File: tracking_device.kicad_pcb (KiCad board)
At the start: 4 copper layers, 74.2 x 35 mm, 74 parts, among them J1 USB_OTG, J2 CONN_COAXIAL, J3 JST-PH, J4 Micro_SD_Connector, J5 CONN_01X03, J6 CONN_01X06, J7 CONN_01X03, J8 SMA, Q1 PMGD280UN, SW1 SW_Push, U1 RClamp0503F, U2 LDK220M30R, U3 MCP73831, U4 MAX-M8, U5 STC3100, U6 STM32L476RG, U7 RFM95W, Y1 ABS07-120-32.768kHz-T

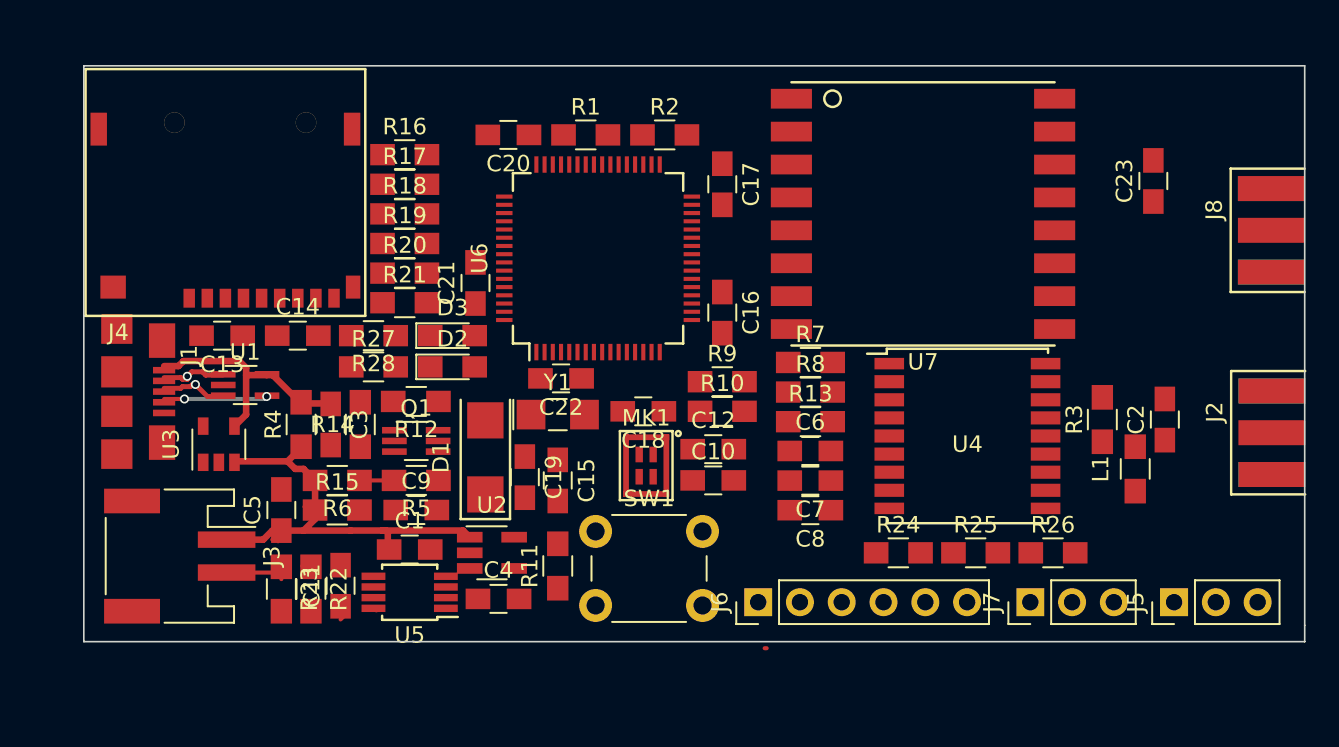
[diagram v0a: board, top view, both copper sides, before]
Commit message: Version sent out for fabrication
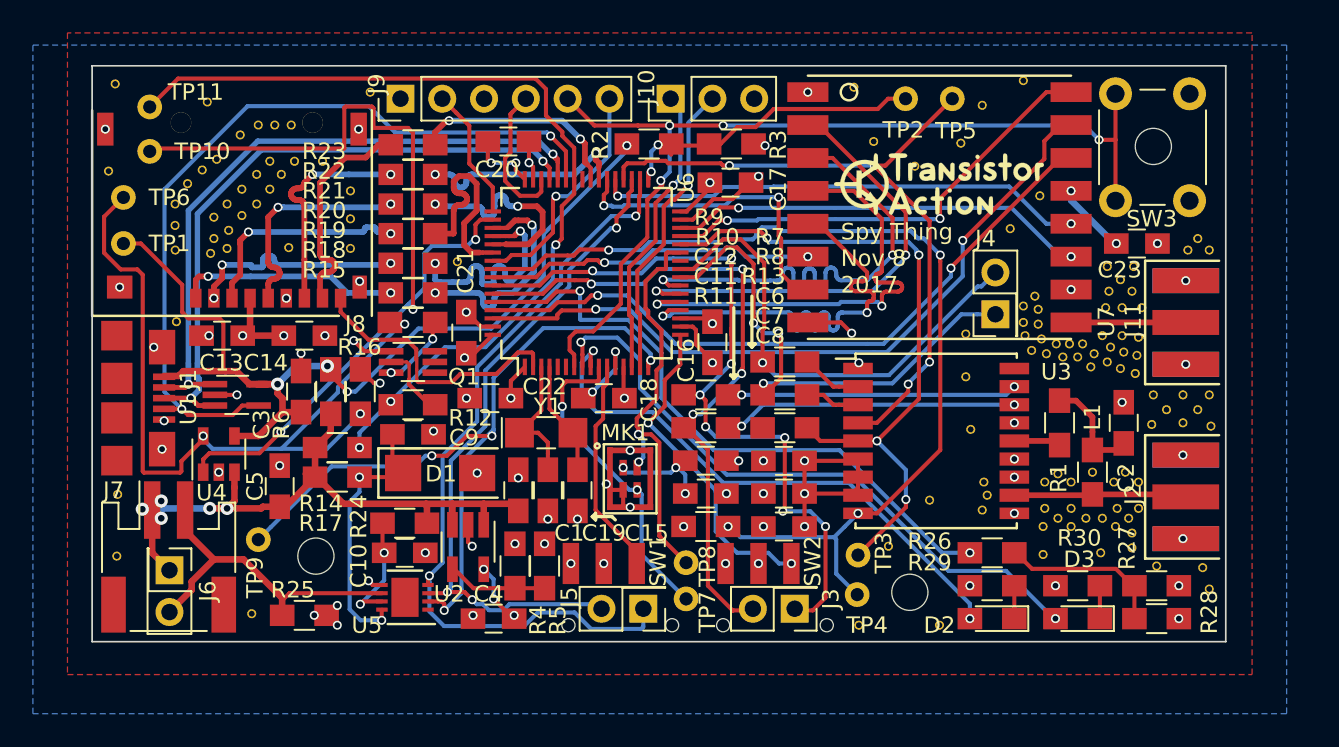
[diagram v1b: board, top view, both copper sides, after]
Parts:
- added ?: , tracking_device:VIA_0.35mm_0.55mm, F.Cu at (97.6, 95.5)
- added ?: , tracking_device:VIA_0.35mm_0.55mm, F.Cu at (155.8, 92.2)
- added ?: , tracking_device:VIA_0.35mm_0.55mm, F.Cu at (154.3, 93.7)
- added ?: , tracking_device:VIA_0.35mm_0.55mm, F.Cu at (154.1, 94.7)
- added ?: , tracking_device:VIA_0.35mm_0.55mm, F.Cu at (153.2, 98.3)
- added ?: , tracking_device:VIA_0.35mm_0.55mm, F.Cu at (152.4, 97.7)
- added ?: , tracking_device:VIA_0.35mm_0.55mm, F.Cu at (151.5, 97.7)
- added ?: , tracking_device:VIA_0.35mm_0.55mm, F.Cu at (150.5, 97.5)
- added ?: , tracking_device:VIA_0.35mm_0.55mm, F.Cu at (149.6, 97.3)
- added ?: , tracking_device:VIA_0.35mm_0.55mm, F.Cu at (149.2, 96.4)
- added ?: , tracking_device:VIA_0.35mm_0.55mm, F.Cu at (149.1, 95.6)
- added ?: , tracking_device:VIA_0.35mm_0.55mm, F.Cu at (149.1, 94.6)
- added ?: , tracking_device:VIA_0.35mm_0.55mm, F.Cu at (155.0, 93.0)
- added ?: , tracking_device:VIA_0.35mm_0.55mm, F.Cu at (149.8, 94.0)
- added ?: , tracking_device:VIA_0.35mm_0.55mm, F.Cu at (150.0, 94.8)
- added ?: , tracking_device:VIA_0.35mm_0.55mm, F.Cu at (150.0, 95.7)
- added ?: , tracking_device:VIA_0.35mm_0.55mm, F.Cu at (150.2, 96.6)
- added ?: , tracking_device:VIA_0.35mm_0.55mm, F.Cu at (151.1, 96.9)
- added ?: , tracking_device:VIA_0.35mm_0.55mm, F.Cu at (151.9, 96.9)
- added ?: , tracking_device:VIA_0.35mm_0.55mm, F.Cu at (152.7, 96.9)
- added ?: , tracking_device:VIA_0.35mm_0.55mm, F.Cu at (155.0, 98.4)
- added ?: , tracking_device:VIA_0.35mm_0.55mm, F.Cu at (153.4, 97.5)
- added ?: , tracking_device:VIA_0.35mm_0.55mm, F.Cu at (154.2, 98.0)
- added ?: , tracking_device:VIA_0.35mm_0.55mm, F.Cu at (155.7, 93.7)
- added ?: , tracking_device:VIA_0.35mm_0.55mm, F.Cu at (155.9, 98.7)
- added ?: , tracking_device:VIA_0.35mm_0.55mm, F.Cu at (154.4, 97.1)
- added ?: , tracking_device:VIA_0.35mm_0.55mm, F.Cu at (153.9, 96.4)
- added ?: , tracking_device:VIA_0.35mm_0.55mm, F.Cu at (155.2, 97.4)
- added ?: , tracking_device:VIA_0.35mm_0.55mm, F.Cu at (104.5, 91.0)
- added ?: MOUNTING_HOLE, Mounting_Holes:MountingHole_2.2mm_M2, F.Cu at (106.1, 109.8)
- added ?: MOUNTING_HOLE, Mounting_Holes:MountingHole_2.2mm_M2, F.Cu at (142.2, 112.0)
- added ?: MOUNTING_HOLE, Mounting_Holes:MountingHole_2.2mm_M2, F.Cu at (157.0, 84.9)
- added ?: , tracking_device:VIA_0.35mm_0.55mm, F.Cu at (156.0, 97.6)
- added ?: LOGO, tracking_device:logo_2, F.Cu at (144.0, 87.1)
- added ?: , tracking_device:VIA_0.35mm_0.55mm, F.Cu at (156.1, 96.5)
- added ?: , tracking_device:VIA_0.35mm_0.55mm, F.Cu at (155.1, 96.4)
- added ?: , tracking_device:VIA_0.35mm_0.55mm, F.Cu at (156.3, 94.7)
- added ?: , tracking_device:VIA_0.35mm_0.55mm, F.Cu at (155.1, 94.7)
- added ?: , tracking_device:VIA_0.35mm_0.55mm, F.Cu at (109.4, 81.6)
- added ?: , tracking_device:VIA_0.35mm_0.55mm, F.Cu at (104.6, 83.6)
- added ?: , tracking_device:VIA_0.35mm_0.55mm, F.Cu at (103.6, 83.6)
- added ?: , tracking_device:VIA_0.35mm_0.55mm, F.Cu at (94.0, 109.8)
- added ?: , tracking_device:VIA_0.35mm_0.55mm, F.Cu at (102.6, 83.6)
- added ?: , tracking_device:VIA_0.35mm_0.55mm, F.Cu at (101.5, 84.2)
- added ?: , tracking_device:VIA_0.35mm_0.55mm, F.Cu at (100.1, 85.7)
- added ?: , tracking_device:VIA_0.35mm_0.55mm, F.Cu at (99.2, 86.3)
- added ?: , tracking_device:VIA_0.35mm_0.55mm, F.Cu at (98.3, 87.2)
- added ?: , tracking_device:VIA_0.35mm_0.55mm, F.Cu at (97.5, 88.4)
- added ?: , tracking_device:VIA_0.35mm_0.55mm, F.Cu at (97.5, 89.7)
- added ?: , tracking_device:VIA_0.35mm_0.55mm, F.Cu at (97.5, 91.2)
- added ?: , tracking_device:VIA_0.35mm_0.55mm, F.Cu at (99.7, 91.4)
- added ?: , tracking_device:VIA_0.35mm_0.55mm, F.Cu at (100.7, 91.1)
- added ?: , tracking_device:VIA_0.35mm_0.55mm, F.Cu at (159.7, 100.9)
- added ?: , tracking_device:VIA_0.35mm_0.55mm, F.Cu at (99.9, 90.5)
- added ?: , tracking_device:VIA_0.35mm_0.55mm, F.Cu at (100.8, 90.0)
- added ?: , tracking_device:VIA_0.35mm_0.55mm, F.Cu at (99.9, 89.2)
- added ?: , tracking_device:VIA_0.35mm_0.55mm, F.Cu at (101.6, 89.1)
- added ?: , tracking_device:VIA_0.35mm_0.55mm, F.Cu at (100.7, 88.4)
- added ?: , tracking_device:VIA_0.35mm_0.55mm, F.Cu at (102.5, 88.4)
- added ?: , tracking_device:VIA_0.35mm_0.55mm, F.Cu at (101.6, 87.5)
- added ?: , tracking_device:VIA_0.35mm_0.55mm, F.Cu at (103.3, 87.5)
- added ?: , tracking_device:VIA_0.35mm_0.55mm, F.Cu at (102.5, 86.6)
- added ?: , tracking_device:VIA_0.35mm_0.55mm, F.Cu at (104.0, 86.6)
- added ?: , tracking_device:VIA_0.35mm_0.55mm, F.Cu at (160.4, 100.0)
- added ?: , tracking_device:VIA_0.35mm_0.55mm, F.Cu at (103.3, 85.8)
- added ?: , tracking_device:VIA_0.35mm_0.55mm, F.Cu at (104.8, 85.8)
- added ?: , tracking_device:VIA_0.35mm_0.55mm, F.Cu at (106.5, 85.8)
- added ?: , tracking_device:VIA_0.35mm_0.55mm, F.Cu at (99.5, 82.2)
- added ?: , tracking_device:VIA_0.35mm_0.55mm, F.Cu at (93.5, 86.4)
- added ?: , tracking_device:VIA_0.35mm_0.55mm, F.Cu at (93.9, 81.1)
- added ?: , tracking_device:VIA_0.35mm_0.55mm, F.Cu at (94.0, 106.0)
- added ?: , tracking_device:VIA_0.35mm_0.55mm, F.Cu at (138.8, 81.3)
- added ?: , tracking_device:VIA_0.35mm_0.55mm, F.Cu at (146.6, 82.4)
- added ?: , tracking_device:VIA_0.35mm_0.55mm, F.Cu at (149.1, 80.9)
- added ?: , tracking_device:VIA_0.35mm_0.55mm, F.Cu at (158.8, 100.0)
- added ?: , tracking_device:VIA_0.35mm_0.55mm, F.Cu at (145.3, 84.7)
- added ?: , tracking_device:VIA_0.35mm_0.55mm, F.Cu at (142.5, 86.1)
- added ?: , tracking_device:VIA_0.35mm_0.55mm, F.Cu at (140.0, 84.6)
- added ?: , tracking_device:VIA_0.35mm_0.55mm, F.Cu at (114.7, 91.9)
- added ?: , tracking_device:VIA_0.35mm_0.55mm, F.Cu at (108.2, 89.3)
- added ?: , tracking_device:VIA_0.35mm_0.55mm, F.Cu at (108.2, 91.1)
- added ?: , tracking_device:VIA_0.35mm_0.55mm, F.Cu at (108.2, 87.6)
- added ?: , tracking_device:VIA_0.35mm_0.55mm, F.Cu at (102.2, 113.3)
- added ?: , tracking_device:VIA_0.35mm_0.55mm, F.Cu at (140.9, 109.2)
- added ?: , tracking_device:VIA_0.35mm_0.55mm, F.Cu at (144.0, 114.0)
- added ?: , tracking_device:VIA_0.35mm_0.55mm, F.Cu at (157.0, 100.0)
- added ?: , tracking_device:VIA_0.35mm_0.55mm, F.Cu at (139.1, 114.0)
- added ?: , tracking_device:VIA_0.35mm_0.55mm, F.Cu at (143.4, 106.4)
- added ?: , tracking_device:VIA_0.35mm_0.55mm, F.Cu at (145.9, 102.1)
- added ?: , tracking_device:VIA_0.35mm_0.55mm, F.Cu at (145.6, 98.9)
- added ?: , tracking_device:VIA_0.35mm_0.55mm, F.Cu at (145.6, 96.3)
- added ?: , tracking_device:VIA_0.35mm_0.55mm, F.Cu at (148.3, 89.9)
- added ?: , tracking_device:VIA_0.35mm_0.55mm, F.Cu at (150.1, 87.9)
- added ?: , tracking_device:VIA_0.35mm_0.55mm, F.Cu at (154.2, 92.2)
- added ?: , tracking_device:VIA_0.35mm_0.55mm, F.Cu at (153.8, 109.6)
- added ?: , tracking_device:VIA_0.35mm_0.55mm, F.Cu at (150.3, 109.7)
- added ?: , tracking_device:VIA_0.35mm_0.55mm, F.Cu at (159.7, 90.5)
- added ?: , tracking_device:VIA_0.35mm_0.55mm, F.Cu at (160.4, 111.8)
- added ?: , tracking_device:VIA_0.35mm_0.55mm, F.Cu at (160.0, 110.5)
- added ?: , tracking_device:VIA_0.35mm_0.55mm, F.Cu at (157.2, 110.4)
- added ?: , tracking_device:VIA_0.35mm_0.55mm, F.Cu at (160.5, 101.9)
- added ?: , tracking_device:VIA_0.35mm_0.55mm, F.Cu at (158.8, 101.7)
- added ?: , tracking_device:VIA_0.35mm_0.55mm, F.Cu at (157.8, 100.9)
- added ?: , tracking_device:VIA_0.35mm_0.55mm, F.Cu at (156.9, 101.8)
- added ?: , tracking_device:VIA_0.35mm_0.55mm, F.Cu at (155.7, 109.3)
- added ?: , tracking_device:VIA_0.35mm_0.55mm, F.Cu at (155.7, 108.4)
- added ?: , tracking_device:VIA_0.35mm_0.55mm, F.Cu at (146.6, 107.0)
- added ?: , tracking_device:VIA_0.35mm_0.55mm, F.Cu at (160.4, 91.2)
- added ?: , tracking_device:VIA_0.35mm_0.55mm, F.Cu at (146.7, 105.3)
- added ?: , tracking_device:VIA_0.35mm_0.55mm, F.Cu at (146.9, 106.1)
- added ?: , tracking_device:VIA_0.35mm_0.55mm, F.Cu at (150.3, 108.0)
- added ?: , tracking_device:VIA_0.35mm_0.55mm, F.Cu at (152.0, 108.0)
- added ?: , tracking_device:VIA_0.35mm_0.55mm, F.Cu at (154.7, 108.0)
- added ?: , tracking_device:VIA_0.35mm_0.55mm, F.Cu at (155.5, 107.5)
- added ?: , tracking_device:VIA_0.35mm_0.55mm, F.Cu at (151.2, 107.5)
- added ?: , tracking_device:VIA_0.35mm_0.55mm, F.Cu at (150.4, 106.9)
- added ?: , tracking_device:VIA_0.35mm_0.55mm, F.Cu at (152.0, 106.9)
- added ?: , tracking_device:VIA_0.35mm_0.55mm, F.Cu at (152.9, 107.5)
- added ?: , tracking_device:VIA_0.35mm_0.55mm, F.Cu at (159.1, 91.2)
- added ?: , tracking_device:VIA_0.35mm_0.55mm, F.Cu at (153.3, 104.7)
- added ?: , tracking_device:VIA_0.35mm_0.55mm, F.Cu at (153.9, 107.5)
- added ?: , tracking_device:VIA_0.35mm_0.55mm, F.Cu at (154.8, 106.9)
- added ?: , tracking_device:VIA_0.35mm_0.55mm, F.Cu at (156.1, 106.9)
- added ?: , tracking_device:VIA_0.35mm_0.55mm, F.Cu at (155.3, 104.7)
- added ?: , tracking_device:VIA_0.35mm_0.55mm, F.Cu at (156.1, 105.3)
- added ?: , tracking_device:VIA_0.35mm_0.55mm, F.Cu at (154.6, 105.3)
- added ?: , tracking_device:VIA_0.35mm_0.55mm, F.Cu at (151.2, 104.8)
- added ?: , tracking_device:VIA_0.35mm_0.55mm, F.Cu at (152.0, 105.3)
- added ?: , tracking_device:VIA_0.35mm_0.55mm, F.Cu at (150.4, 105.3)
- added J4: CONN_01X02, tracking_device:Pin_Header_Straight_2x01_Pitch2.54mm, F.Cu at (147.4, 95.1)
- added J6: CONN_01X02, tracking_device:Pin_Header_Straight_2x01_Pitch2.54mm, F.Cu at (97.2, 110.7)
- added J7: JST-PH, tracking_device:JST_PH_S2B-PH-SM4-TB_02x2.00mm_Angled, F.Cu at (93.2, 106.6)
- added R4: 10k, Resistors_SMD:R_0805_HandSoldering, F.Cu at (118.2, 110.4)
- added R5: 5.6k, Resistors_SMD:R_0805_HandSoldering, F.Cu at (120.0, 110.4)
- added SW1: SW_SPDT, tracking_device:CSS-1210TB, F.Cu at (124.6, 111.5)
- added SW2: SW_SPDT, tracking_device:CSS-1210TB, F.Cu at (134.0, 111.5)
- added TP1: TEST, Measurement_Points:Measurement_Point_Round-TH_Small, F.Cu at (94.4, 90.8)
- added TP10: TEST, Measurement_Points:Measurement_Point_Round-TH_Small, F.Cu at (96.0, 85.2)
- added TP11: TEST, Measurement_Points:Measurement_Point_Round-TH_Small, F.Cu at (96.0, 82.5)
- added TP2: TEST, Measurement_Points:Measurement_Point_Round-TH_Small, F.Cu at (141.9, 82.0)
- added TP3: TEST, Measurement_Points:Measurement_Point_Round-TH_Small, F.Cu at (139.1, 109.7)
- added TP4: TEST, Measurement_Points:Measurement_Point_Round-TH_Small, F.Cu at (139.0, 112.1)
- added TP5: TEST, Measurement_Points:Measurement_Point_Round-TH_Small, F.Cu at (144.8, 82.0)
- added TP6: TEST, Measurement_Points:Measurement_Point_Round-TH_Small, F.Cu at (94.4, 88.0)
- added TP7: TEST, Measurement_Points:Measurement_Point_Round-TH_Small, F.Cu at (128.6, 112.4)
- added TP8: TEST, Measurement_Points:Measurement_Point_Round-TH_Small, F.Cu at (128.6, 110.2)
- added TP9: TEST, Measurement_Points:Measurement_Point_Round-TH_Small, F.Cu at (102.6, 108.8)
- J3: value JST-PH -> CONN_01X02; footprint Connectors_JST:JST_PH_S2B-PH-SM4-TB_02x2.00mm_Angled -> tracking_device:Pin_Header_Straight_2x01_Pitch2.54mm
- J5: value CONN_01X03 -> CONN_01X02; footprint Pin_Headers:Pin_Header_Straight_1x03_Pitch2.54mm -> tracking_device:Pin_Header_Straight_2x01_Pitch2.54mm
- R12: renamed from R5; value 100 -> 100 (DNI)
- R14: renamed from R6; value 10k -> 10k (DNI)
- R15: renamed from R12; value 12 -> DNI
- R16: renamed from R14; value 500k -> 12k
- U5: footprint Housings_SSOP:MSOP-8_3x3mm_Pitch0.65mm -> Housings_DFN_QFN:DFN-8-1EP_3x3mm_Pitch0.5mm
- moved R30 45.4 mm to (152.4, 111.6)
- moved D3 41.7 mm to (152.4, 113.6), turned to 180 degrees
- moved R29 39.9 mm to (147.2, 111.6), turned to 180 degrees
- moved J10 37.6 mm to (127.7, 82.0)
- moved J3 37.5 mm to (135.2, 113.0), turned to 180 degrees
- moved J9 37.5 mm to (111.2, 82.0)
- moved SW3 37.5 mm to (154.7, 88.2), turned to 90 degrees
- moved D2 36.2 mm to (147.2, 113.6), turned to 180 degrees
- moved J5 32.3 mm to (126.0, 113.0), turned to 180 degrees
- moved R27 11.2 mm to (157.2, 111.6)
- moved R23 9.61 mm to (112.0, 84.8)
- moved R11 9.31 mm to (129.8, 108.0), turned to 0 degrees
- moved R18 8.41 mm to (112.0, 93.8)
- moved J11 7.64 mm to (161.0, 95.6)
- moved C1 7.52 mm to (118.4, 105.8), turned to 270 degrees
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- renumbered C11 to C10, C10 to C11, J7 to J10, J8 to J11, J4 to J8, J6 to J9, R3 to R1, R15 to R17, R16 to R18, R17 to R19, R1 to R2, R18 to R20, R19 to R21, R20 to R22, R21 to R23, R22 to R24, R23 to R25, R24 to R26, R25 to R27, R26 to R28, R27 to R29, R2 to R3, R28 to R30, R4 to R6, SW1 to SW3, U4 to U3, U3 to U4
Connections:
- C1 pad 1: /VBAT -> GND
- C1 pad 2: GND -> /VBAT
- J3 pad 1: /VBAT -> /GPS_I2C_SCL
- J3 pad 2: Net-(J3-Pad2) -> /GPS_I2C_SDA
- J5 pad 1: VDD -> /PMIC_I2C_SCL
- J5 pad 2: Net-(J5-Pad2) -> /PMIC_I2C_SDA
- Q1 pad 1: Net-(Q1-Pad1) -> GND
- R15 pad 1: GND -> Net-(Q1-Pad3)
- R15 pad 2: Net-(Q1-Pad1) -> Net-(R15-Pad2)
- R16 pad 1: Net-(Q1-Pad3) -> Net-(R15-Pad2)
- R25 pad 1: Net-(J3-Pad2) -> Net-(J6-Pad2)
- R26 pad 2: Net-(J5-Pad2) -> Net-(R26-Pad2)
- R27 pad 1: Net-(J5-Pad2) -> Net-(R26-Pad2)
- R28 pad 1: Net-(J5-Pad2) -> Net-(R26-Pad2)
- U3 pad 4: /GPS_EXTINT -> /GPS_TIMEPULSE
- U4 pad 5: Net-(Q1-Pad3) -> Net-(R15-Pad2)
- U5 pad 6: Net-(J3-Pad2) -> Net-(J6-Pad2)
- U6 pad 11: Net-(U6-Pad11) -> /Microcontroller/SWITCH_1
- U6 pad 17: Net-(U6-Pad17) -> /Microcontroller/SWITCH_2
- U6 pad 26: /PMIC_FAST -> Net-(U6-Pad26)
- U6 pad 28: Net-(U6-Pad28) -> /GPS_EXTINT
- U6 pad 33: Net-(U6-Pad33) -> /VUSB_DET
- U6 pad 36: Net-(U6-Pad36) -> /GPS_TIMEPULSE
- U6 pad 42: Net-(U6-Pad42) -> /PMIC_FAST
- U6 pad 56: Net-(U6-Pad56) -> /GPS_RESET_N
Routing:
- net /GPS_RESET_N: track 0.00 -> 60.4 mm, vias 0 -> 4
- net /Microcontroller/NRST: track 0.00 -> 59.0 mm, vias 0 -> 4
- net /PMIC_STAT: track 0.00 -> 57.3 mm, vias 0 -> 3
- net /PMIC_FAST: track 2.10 -> 54.5 mm, vias 0 -> 3
- net VDD: track 0.00 -> 48.3 mm, vias 0 -> 24
- net /PMIC_I2C_SCL: track 0.00 -> 48.3 mm, vias 0 -> 2
- net /GPS_I2C_SCL: track 0.00 -> 47.0 mm, vias 0 -> 8
- net Net-(R15-Pad2): track 0.00 -> 46.7 mm, vias 0 -> 3
- net /LSE_CLK: track 0.00 -> 46.5 mm, vias 0 -> 4
- net GND: track 0.00 -> 44.7 mm, vias 0 -> 65
- net /SX1272/DIO1: track 0.00 -> 44.2 mm, vias 0 -> 2
- net /USB_ID: track 6.30 -> 49.3 mm
- net /VUSB: track 15.0 -> 57.9 mm, vias 0 -> 4
- net /GPS_TIMEPULSE: track 0.00 -> 42.2 mm, vias 0 -> 4
- net /SX1272/DIO0: track 0.00 -> 41.7 mm, vias 0 -> 2
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- added copper zone on B.Cu, net GND
- added copper zone on F.Cu, net GND
- added copper zone on Ground, net GND
- added copper zone on Power, net VDD
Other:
- board size 74.2 x 35 mm -> 68.9 x 35 mm
- net class 50 ohm: clearance 0.2 -> 0.16
- net class Default: clearance 0.25 -> 0.16
- net class USB: clearance 0.15 -> 0.16
- net class power: clearance 0.3 -> 0.16
- rule trace_clearance: 0.25 -> 0.16
- board text added: "Spy Thing Nov 8 2017"
